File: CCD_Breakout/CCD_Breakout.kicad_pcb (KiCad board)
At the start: 2 copper layers, 16 x 76.5 mm, 9 parts, among them Q1 PNP, U1 ILX511

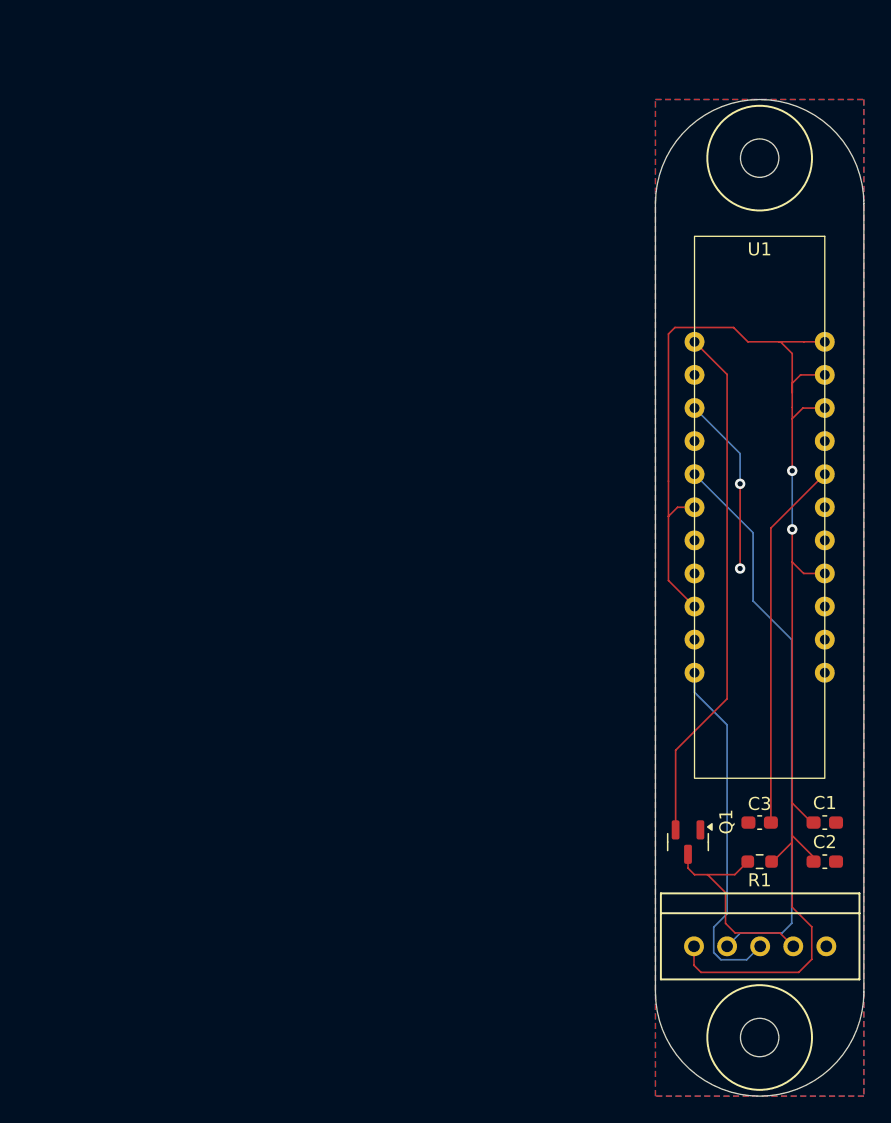
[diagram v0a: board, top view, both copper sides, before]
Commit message: cat
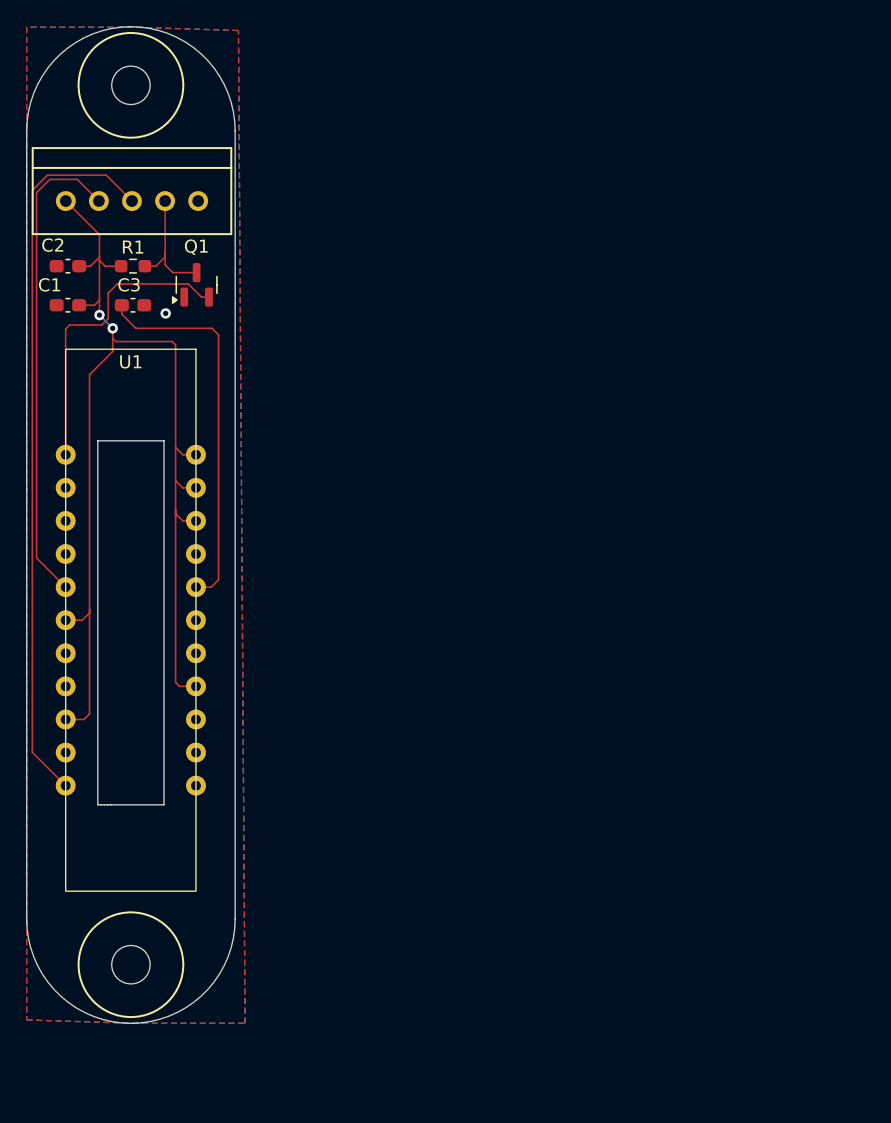
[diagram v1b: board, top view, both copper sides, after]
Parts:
- moved Conn1 74.8 mm to (66.2, 41.5)
- moved C2 73.9 mm to (66.4, 46.5), turned to 180 degrees
- moved C1 70.4 mm to (66.4, 49.5), turned to 180 degrees
- moved R1 66.4 mm to (71.4, 46.5), turned to 0 degrees
- moved C3 62.4 mm to (71.4, 49.5), turned to 180 degrees
- moved Q1 57.0 mm to (76.3, 48.0), turned to 90 degrees
- moved U1 49.0 mm to (76.2, 52.9)
- moved H1 48.6 mm to (71.2, 32.7)
- moved H2 48.6 mm to (71.2, 100.2)
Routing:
- net ROG: track 27.2 -> 55.7 mm
- net +5V: track 112.8 -> 90.6 mm
- net Net-(Q1-B): track 40.1 -> 23.6 mm
- net GND: track 13.8 -> 0.00 mm, vias 2 -> 1
- net Vout: track 16.5 -> 9.77 mm
- net CLK: track 43.3 -> 37.1 mm
- net Net-(U1-VGG): track 28.5 -> 29.5 mm
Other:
- outline, holes or cut-outs redrawn
